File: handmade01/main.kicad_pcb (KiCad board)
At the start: 2 copper layers, 64.8 x 70.1 mm, 69 parts, among them CON1 MicroSD, CON2 MicroSD, J1 JACK_TRS_6PINS, P1 VOLUMN, P4 USB_OTG, P6 UART_DEBUG, Q1 1AM, SW1 Power, SW10 R, SW11 A, SW12 B, SW13 X, SW14 Y, SW2 Reset, SW3 UP, SW4 Down, SW5 Left, SW6 Right, SW7 Select, SW8 Start, SW9 L, U1 PCM5102A, U2 PAM8403, U3 IPS_2.4_240x320_ST7789V, U4 CM3354, U5 TPS71718

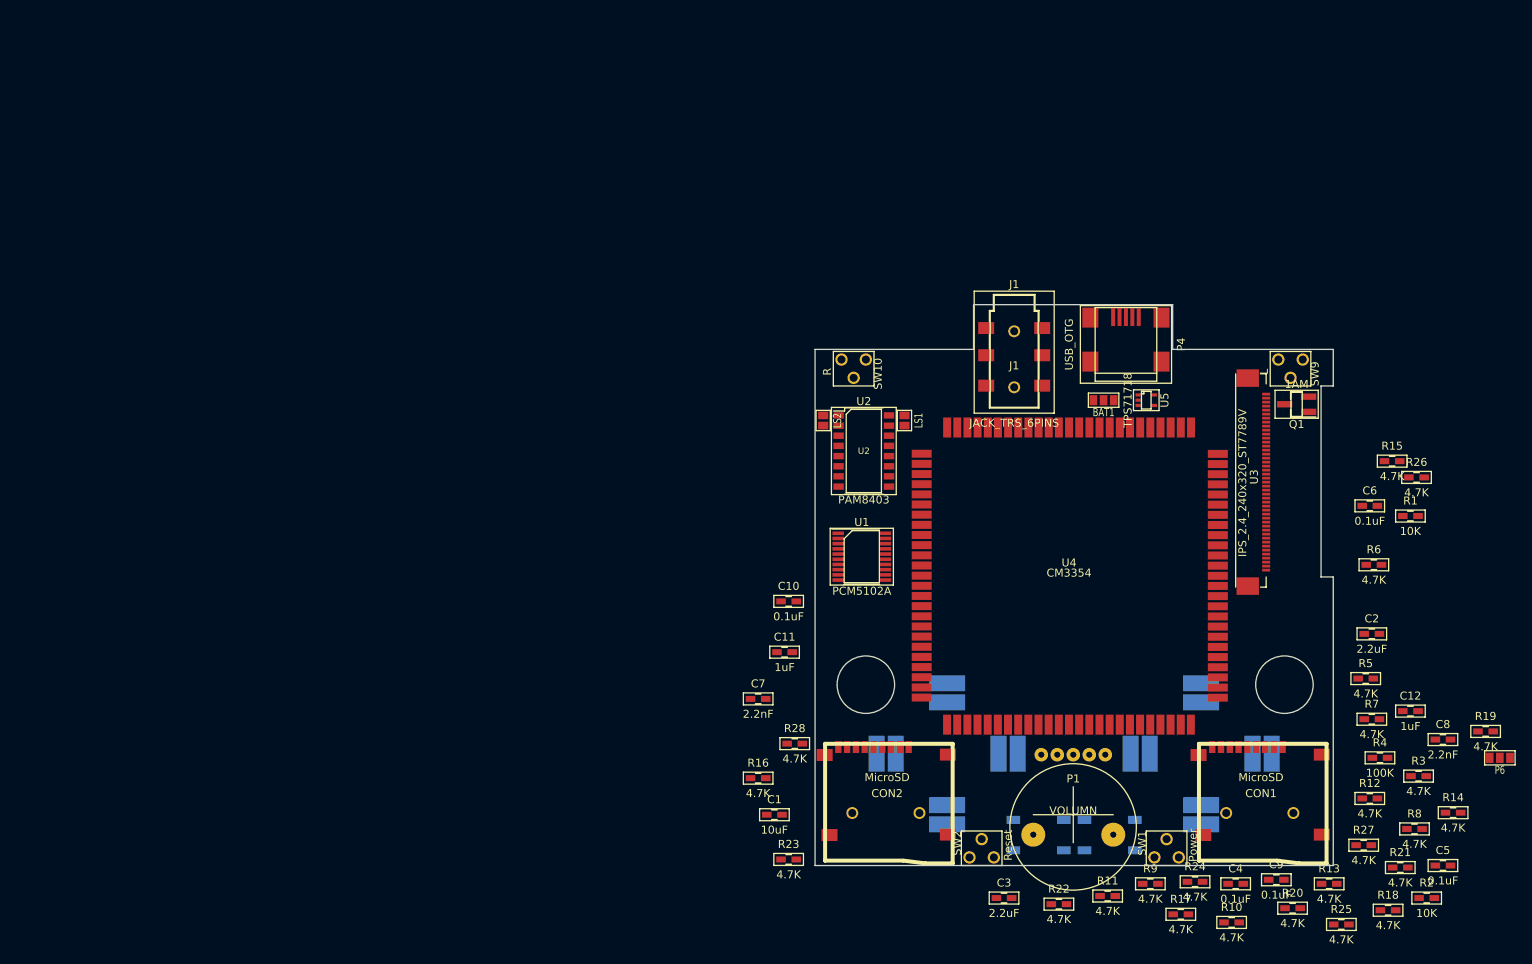
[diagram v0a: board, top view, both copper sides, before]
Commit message: 20171208
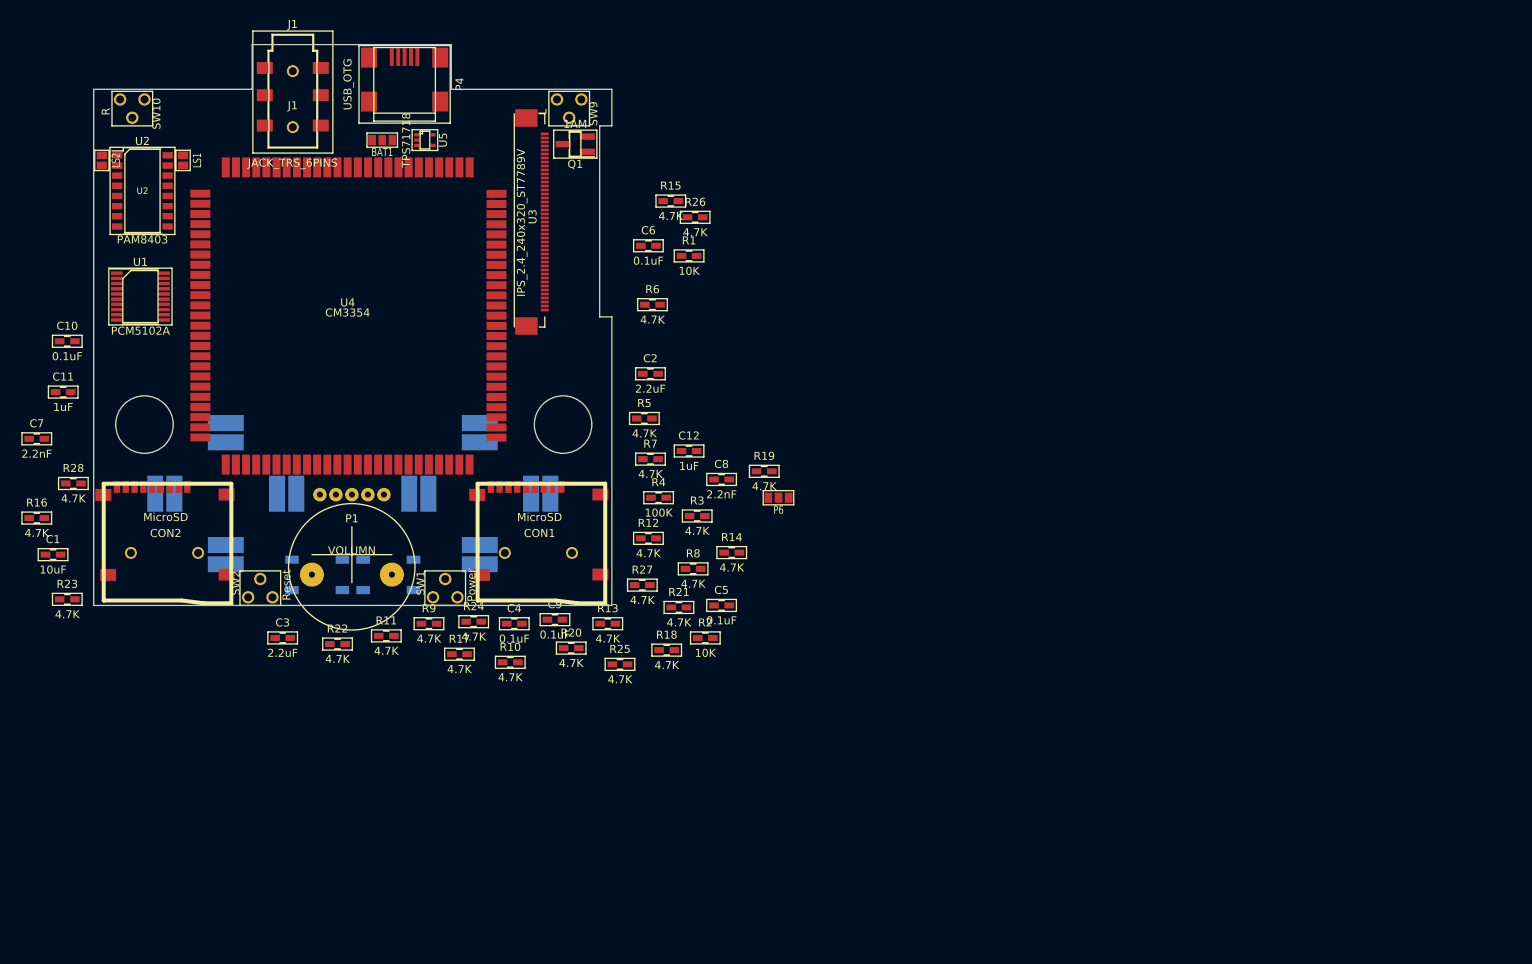
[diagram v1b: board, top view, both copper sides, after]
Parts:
- moved BAT1 95.9 mm to (146.6, 79.5)
- moved C1 95.9 mm to (105.4, 131.3)
- moved C3 95.9 mm to (134.1, 141.7)
- moved C5 95.9 mm to (189.0, 137.7)
- moved C6 95.9 mm to (179.8, 92.7)
- moved CON1 95.9 mm to (170.2, 133.6)
- moved LS1 95.9 mm to (121.7, 82.0)
- moved P1 95.9 mm to (142.7, 131.3)
- moved Q1 95.9 mm to (170.7, 80.0)
- moved R12 95.9 mm to (179.8, 129.3)
- moved R13 95.9 mm to (174.8, 140.0)
- moved R18 95.9 mm to (182.1, 143.3)
- moved R19 95.9 mm to (194.3, 120.9)
- moved R20 95.9 mm to (170.2, 143.0)
- moved R21 95.9 mm to (183.6, 137.9)
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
